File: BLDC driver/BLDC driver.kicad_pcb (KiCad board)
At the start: 4 copper layers, 75 x 50 mm, 40 parts, among them J1 Screw_Terminal_01x02, J2 Screw_Terminal_01x03, J3 Conn_02x06_Counter_Clockwise, J4 Izlaz ocitavanje struje, Q1 N0436N, Q2 N0436N, Q3 N0436N, Q4 N0436N, Q5 N0436N, Q6 N0436N, U1 MCP8027T-H/Y4X

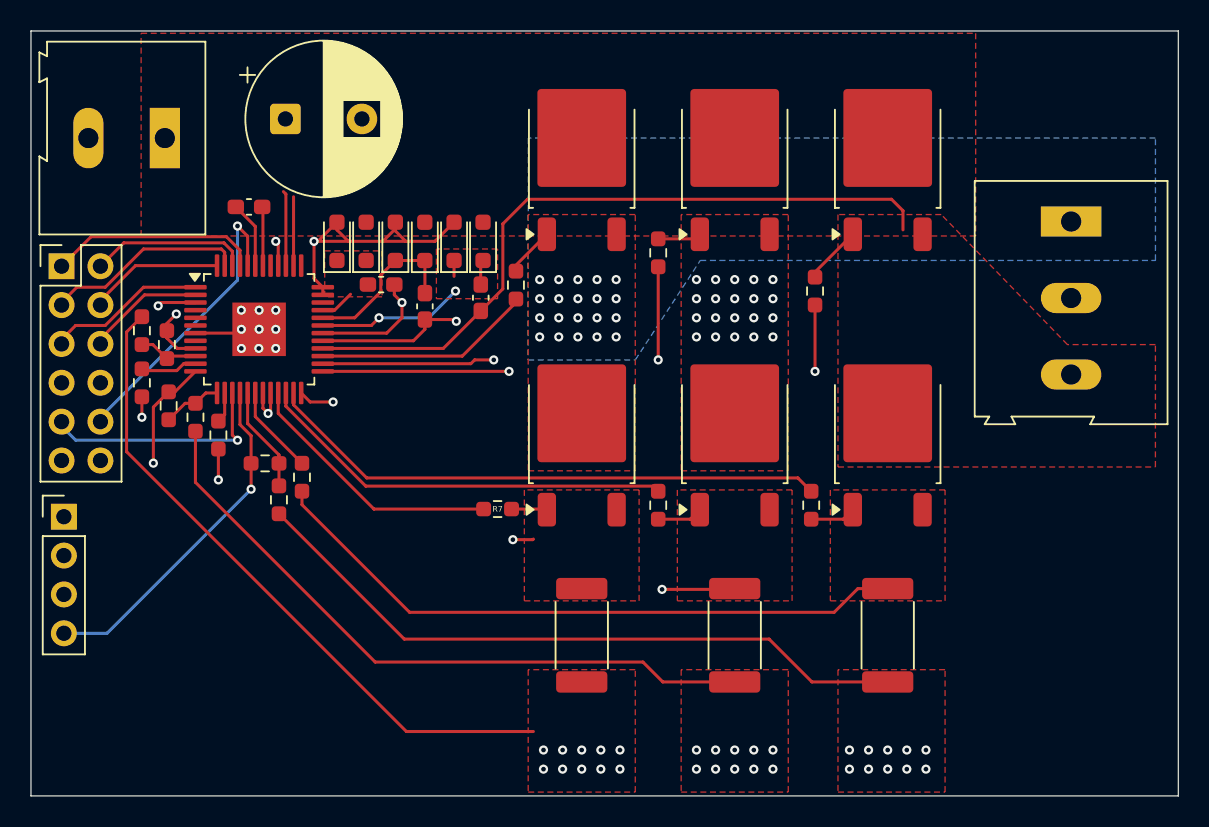
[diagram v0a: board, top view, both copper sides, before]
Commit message: Dodadi kondenzatori, vratiti u slucaju greske
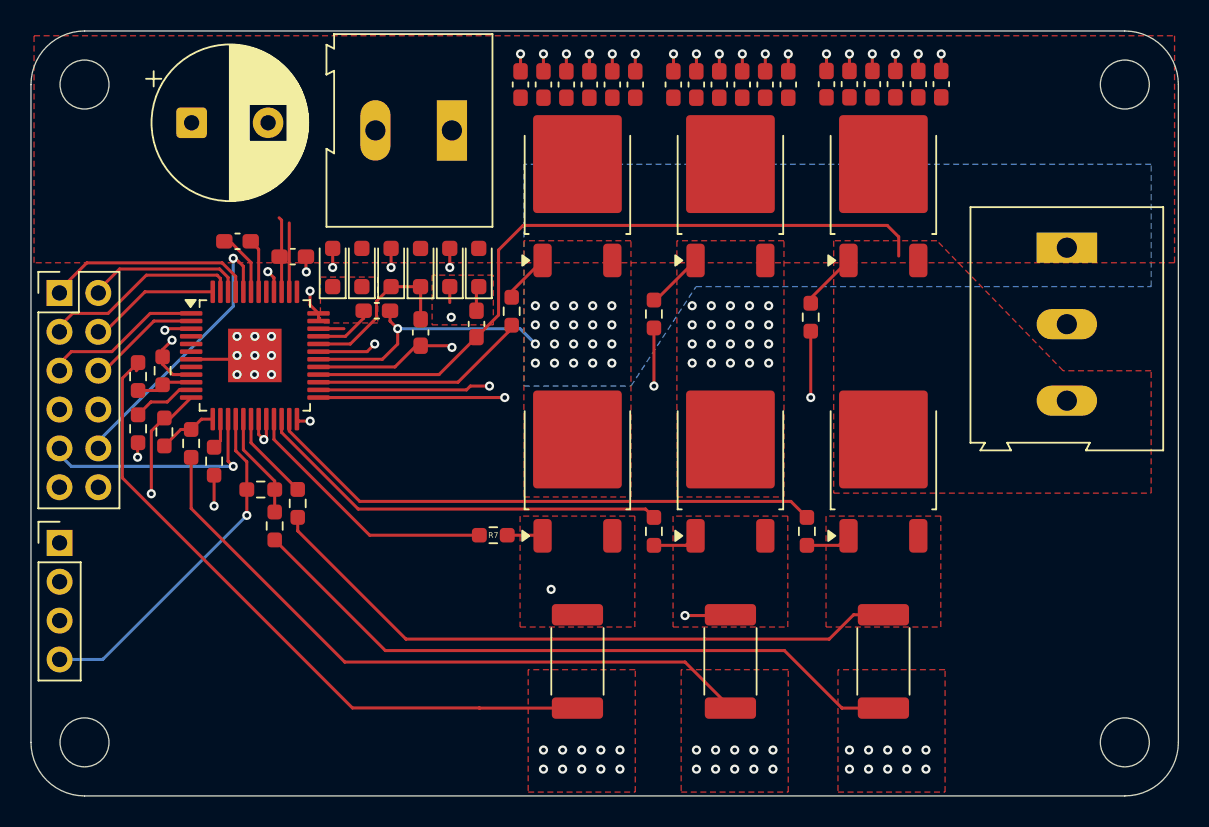
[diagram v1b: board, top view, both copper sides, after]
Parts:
- added C10: 470n, Capacitor_SMD:C_0603_1608Metric_Pad1.08x0.95mm_HandSolder, F.Cu at (160.5, 62.2)
- added C11: 470n, Capacitor_SMD:C_0603_1608Metric_Pad1.08x0.95mm_HandSolder, F.Cu at (162.0, 62.2)
- added C12: 470n, Capacitor_SMD:C_0603_1608Metric_Pad1.08x0.95mm_HandSolder, F.Cu at (163.5, 62.2)
- added C13: 470n, Capacitor_SMD:C_0603_1608Metric_Pad1.08x0.95mm_HandSolder, F.Cu at (166.0, 62.2)
- added C14: 470n, Capacitor_SMD:C_0603_1608Metric_Pad1.08x0.95mm_HandSolder, F.Cu at (167.5, 62.2)
- added C15: 470n, Capacitor_SMD:C_0603_1608Metric_Pad1.08x0.95mm_HandSolder, F.Cu at (169.0, 62.2)
- added C16: 470n, Capacitor_SMD:C_0603_1608Metric_Pad1.08x0.95mm_HandSolder, F.Cu at (170.5, 62.2)
- added C17: 470n, Capacitor_SMD:C_0603_1608Metric_Pad1.08x0.95mm_HandSolder, F.Cu at (172.0, 62.2)
- added C18: 470n, Capacitor_SMD:C_0603_1608Metric_Pad1.08x0.95mm_HandSolder, F.Cu at (173.5, 62.2)
- added C19: 470n, Capacitor_SMD:C_0603_1608Metric_Pad1.08x0.95mm_HandSolder, F.Cu at (182.0, 62.2)
- added C20: 470n, Capacitor_SMD:C_0603_1608Metric_Pad1.08x0.95mm_HandSolder, F.Cu at (183.5, 62.2)
- added C21: 470n, Capacitor_SMD:C_0603_1608Metric_Pad1.08x0.95mm_HandSolder, F.Cu at (176.0, 62.2)
- added C22: 470n, Capacitor_SMD:C_0603_1608Metric_Pad1.08x0.95mm_HandSolder, F.Cu at (177.5, 62.2)
- added C23: 470n, Capacitor_SMD:C_0603_1608Metric_Pad1.08x0.95mm_HandSolder, F.Cu at (179.0, 62.2)
- added C24: 470n, Capacitor_SMD:C_0603_1608Metric_Pad1.08x0.95mm_HandSolder, F.Cu at (180.5, 62.2)
- added C6: 470n, Capacitor_SMD:C_0603_1608Metric_Pad1.08x0.95mm_HandSolder, F.Cu at (141.1, 73.5)
- added C7: 470n, Capacitor_SMD:C_0603_1608Metric_Pad1.08x0.95mm_HandSolder, F.Cu at (156.0, 62.2)
- added C8: 470n, Capacitor_SMD:C_0603_1608Metric_Pad1.08x0.95mm_HandSolder, F.Cu at (157.5, 62.2)
- added C9: 470n, Capacitor_SMD:C_0603_1608Metric_Pad1.08x0.95mm_HandSolder, F.Cu at (159.0, 62.2)
- added H1: MountingHole, MountingHole:MountingHole_3.2mm_M3, F.Cu at (127.5, 62.2)
- added H2: MountingHole, MountingHole:MountingHole_3.2mm_M3, F.Cu at (195.5, 62.2)
- added H3: MountingHole, MountingHole:MountingHole_3.2mm_M3, F.Cu at (195.5, 105.2)
- added H4: MountingHole, MountingHole:MountingHole_3.2mm_M3, F.Cu at (127.5, 105.2)
- moved J1 18.8 mm to (151.5, 65.2)
- moved C5 6.14 mm to (134.5, 64.8)
- moved R5 4.01 mm to (164.7, 77.2)
- moved R11 3.01 mm to (131.0, 84.8)
- moved R13 3.01 mm to (131.0, 81.3)
- moved C4 2.37 mm to (137.5, 72.5)
- moved J3 1.75 mm to (125.9, 75.9)
- moved D2 1.73 mm to (149.5, 74.2)
- moved J2 1.73 mm to (191.7, 72.9)
- moved R12 1.73 mm to (141.4, 89.6)
- moved R14 1.73 mm to (139.9, 91.1)
- moved R4 1.73 mm to (155.4, 77.1)
- moved R9 1.73 mm to (136.0, 86.9)
- moved C1 1.73 mm to (149.5, 78.5)
- moved C2 1.73 mm to (153.1, 77.9)
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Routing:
- net GND: track 161.4 -> 166.1 mm, vias 42 -> 64
- net Net-(U1-HSB): track 28.1 -> 25.8 mm
- net Net-(D1-K): track 2.24 -> 3.93 mm
- net unconnected-(U1-+12V-Pad34): track 0.00 -> 1.67 mm
- net Net-(Q2-G): track 3.37 -> 4.35 mm
- net PWM2H: track 8.86 -> 7.93 mm
- net Net-(Q4-S): track 31.0 -> 31.8 mm
- net DE2: track 19.4 -> 18.7 mm
- net PWM1H: track 7.86 -> 7.25 mm
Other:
- outline, holes or cut-outs redrawn
